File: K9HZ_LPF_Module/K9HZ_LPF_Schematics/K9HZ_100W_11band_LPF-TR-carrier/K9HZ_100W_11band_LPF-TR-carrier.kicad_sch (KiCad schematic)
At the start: 12 parts, among them J22.1 ANTENNA, J22.2 TRANSMIT, J23.1 RECEIVE, J23.2 TR CTL, K1 HF41F/12-ZS, K2 HF41F/12-ZS, Q1 BS170

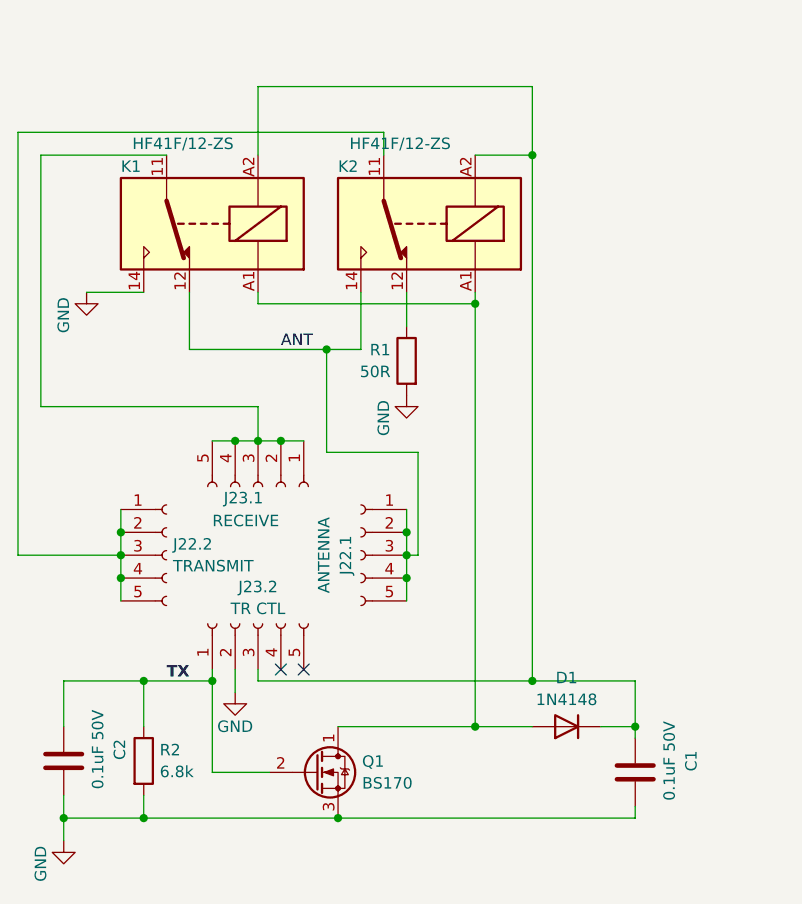
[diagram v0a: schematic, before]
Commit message: ATU Update
ATU Update
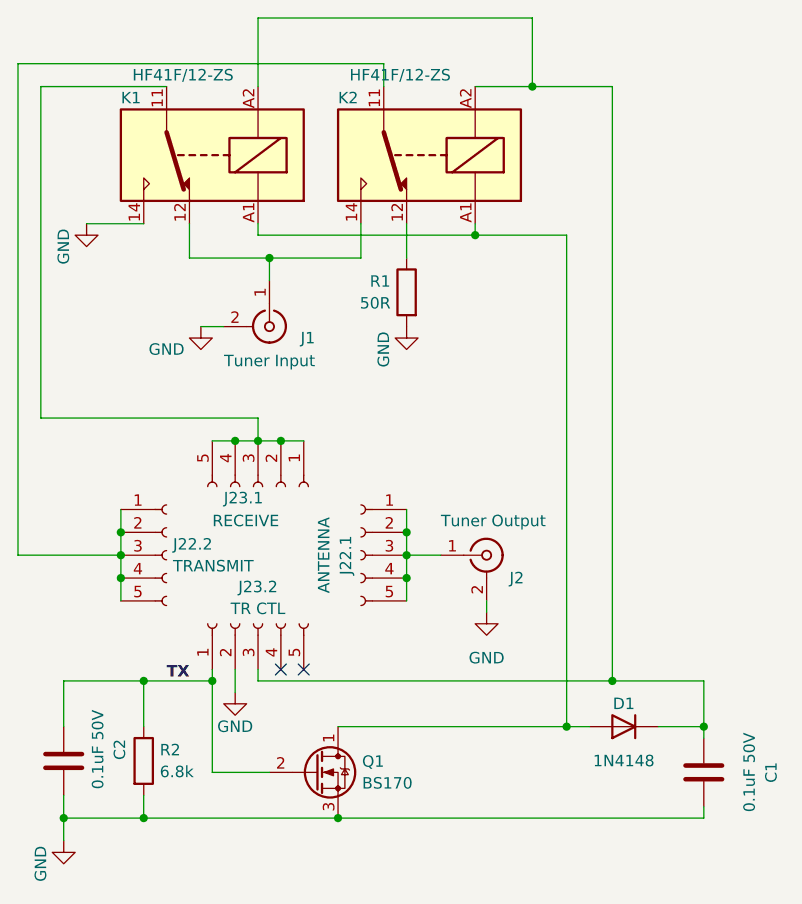
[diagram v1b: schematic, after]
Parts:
- added J1: Tuner Input, Connector_Coaxial:SMA_Amphenol_901-144_Vertical, symbol Connector:Conn_Coaxial
- added J2: Tuner Output, Connector_Coaxial:SMA_Amphenol_901-144_Vertical, symbol Connector:Conn_Coaxial
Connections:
- net GND: now also J1.2 (Ext), J2.2 (Ext)
- net ANT: no longer names the net of J22.1.1 (Pin_1), J22.1.2 (Pin_2), J22.1.3 (Pin_3), J22.1.4 (Pin_4), J22.1.5 (Pin_5)
- net ANT: now also J2.1 (In); no longer K1.12, K2.14
- new net: J1.1 (In), K1.12, K2.14
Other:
- moved on the sheet: C1, D1, K1, K2, R1
